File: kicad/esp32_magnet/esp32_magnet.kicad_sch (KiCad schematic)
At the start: 1 part, among them U1 ESP32-S3-WROOM-1

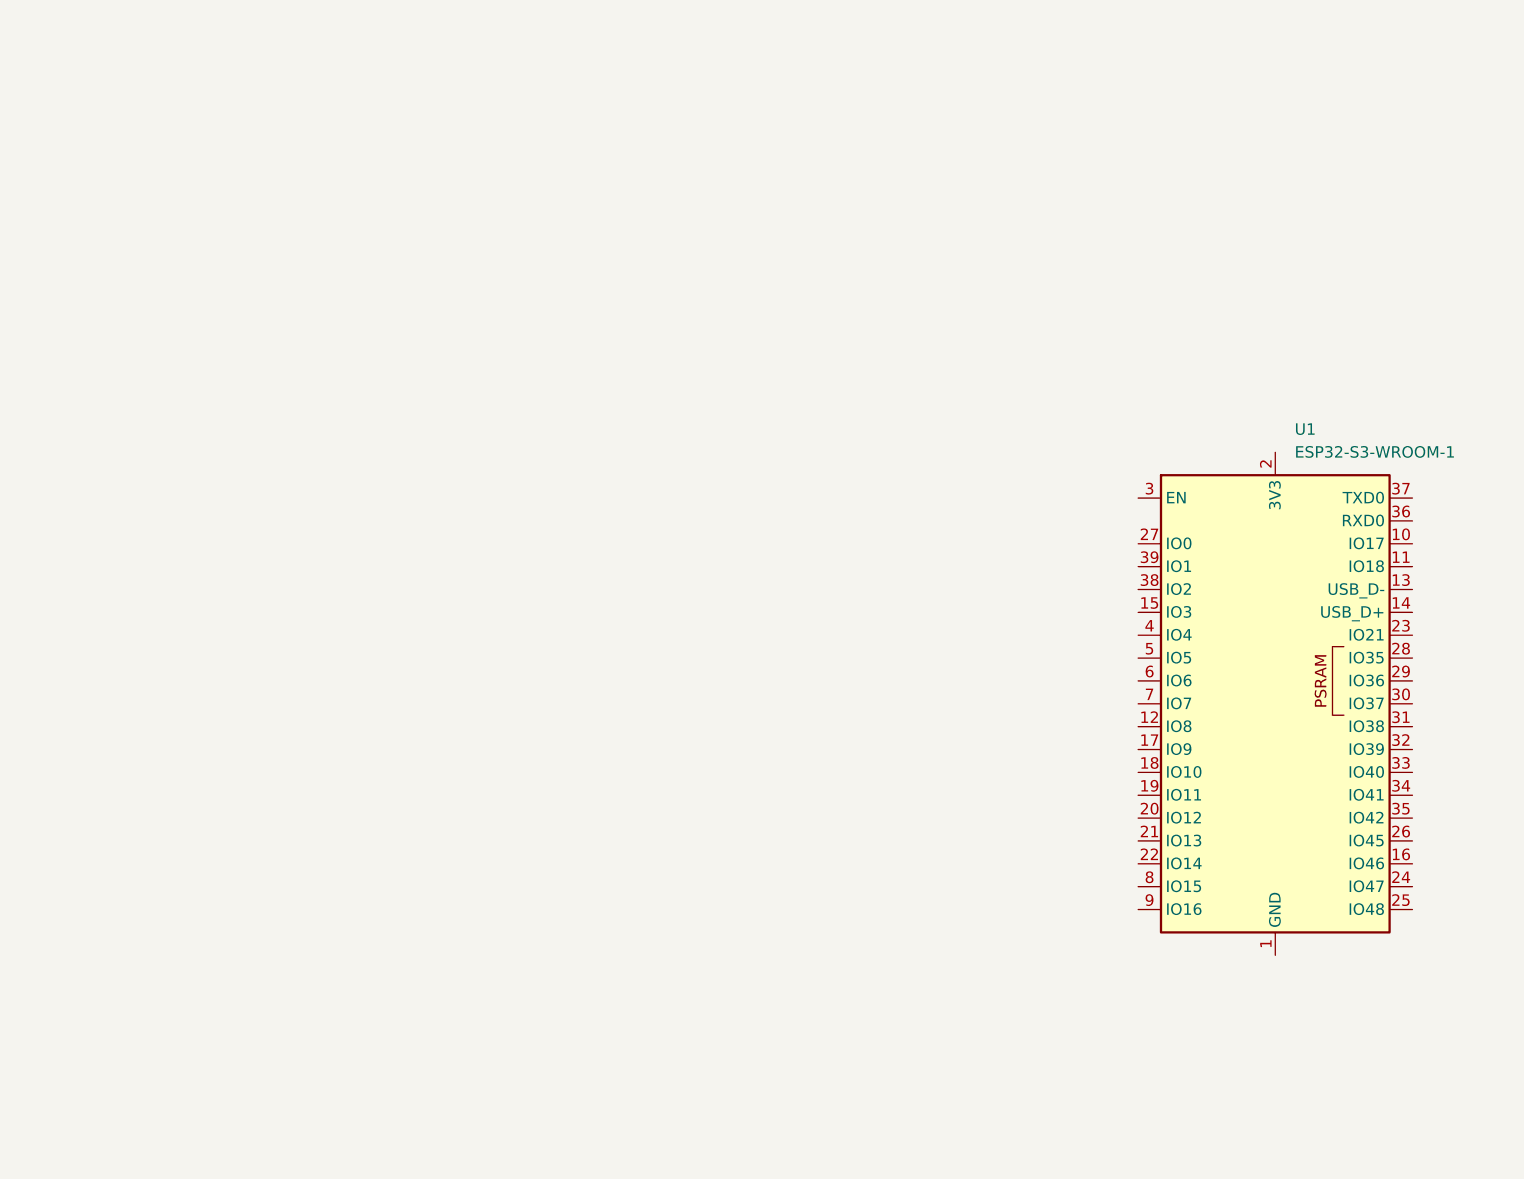
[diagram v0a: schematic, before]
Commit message: fix(kicad):esp32 base sch
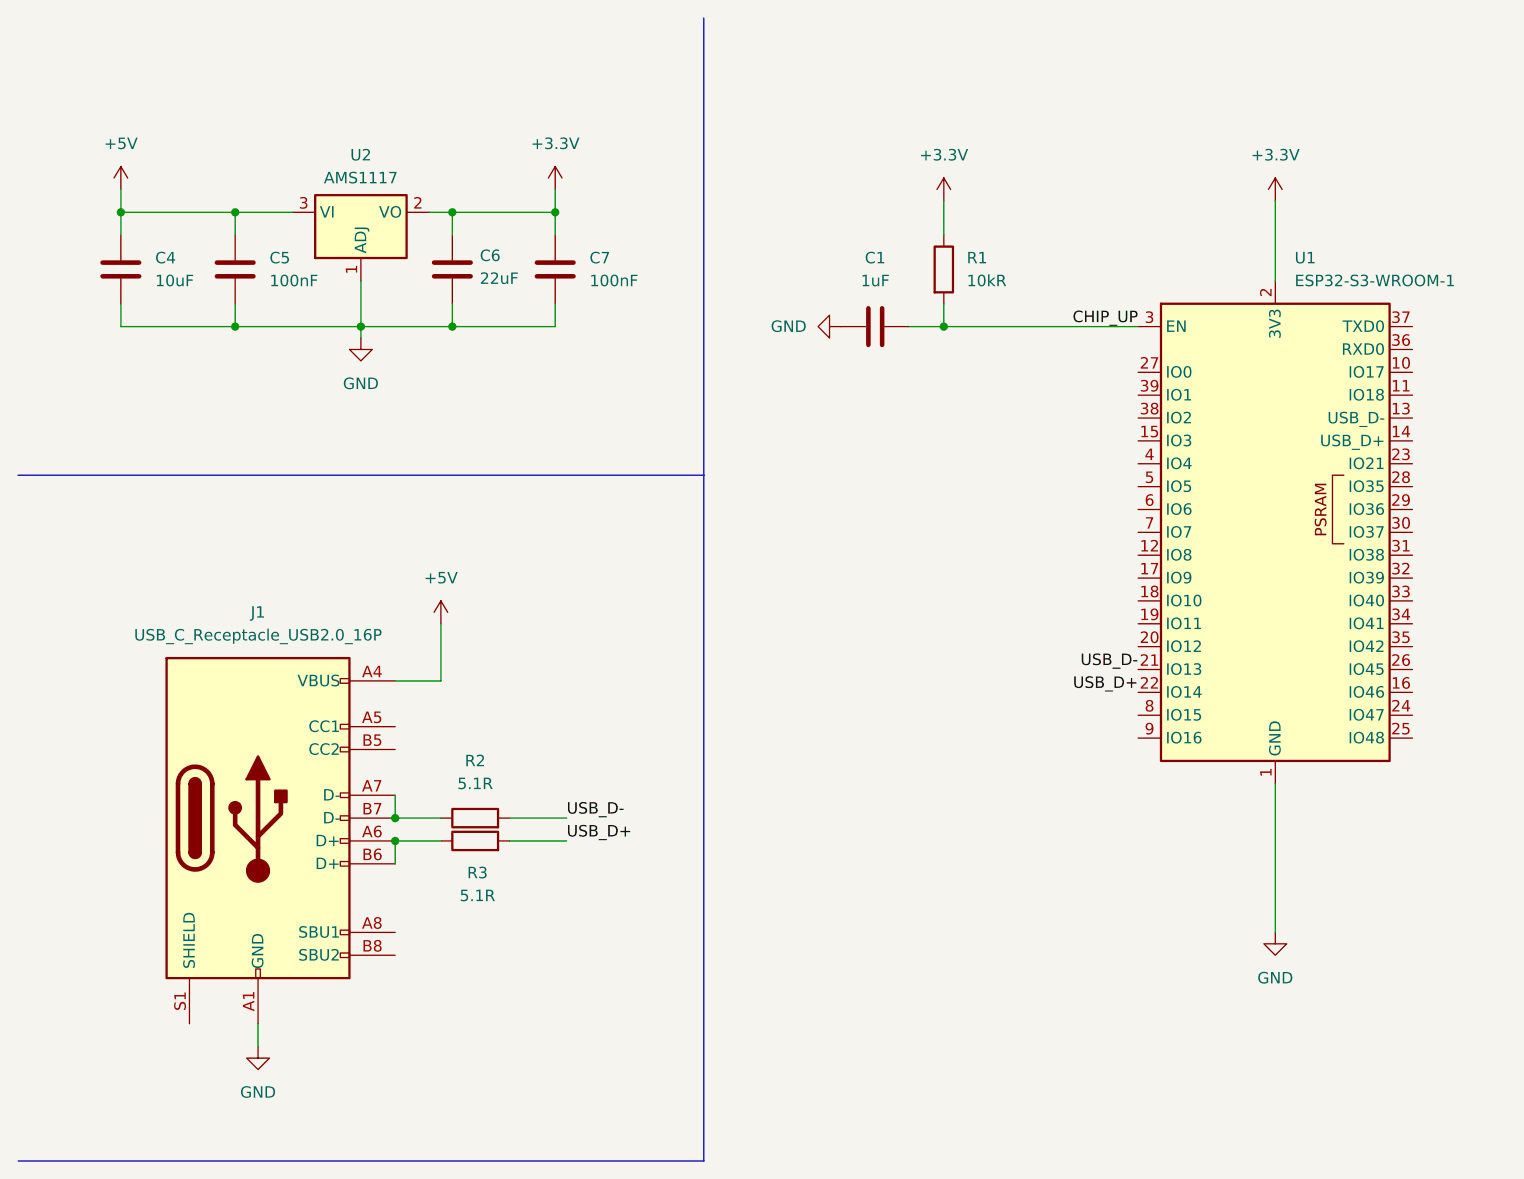
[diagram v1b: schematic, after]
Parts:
- added C1: 1uF, Capacitor_SMD:C_0603_1608Metric, symbol Device:C
- added C4: 10uF, Capacitor_SMD:C_0603_1608Metric, symbol Device:C
- added C5, C7: 100nF, Capacitor_SMD:C_0603_1608Metric, symbol Device:C
- added C6: 22uF, Capacitor_SMD:C_0603_1608Metric, symbol Device:C
- added J1: USB_C_Receptacle_USB2.0_16P, Connector_USB:USB_C_Receptacle_GCT_USB4105-xx-A_16P_TopMnt_Horizontal, symbol Connector:USB_C_Receptacle_USB2.0_16P
- added R1: 10kR, Resistor_SMD:R_1206_3216Metric, symbol Device:R
- added R2, R3: 5.1R, Resistor_SMD:R_1206_3216Metric, symbol Device:R
- added U2: AMS1117, Package_TO_SOT_SMD:SOT-223-3_TabPin2, symbol Regulator_Linear:AMS1117
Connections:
- net GND: now reaches U1.1 (GND), U1.40 (GND), U1.41 (GND)
- net GND: now also C1.1, C4.2, C5.2, C6.2, C7.2, J1.A1 (GND), J1.A12 (GND), J1.B1 (GND), J1.B12 (GND), U2.1 (ADJ)
- net +3.3V: now reaches U1.2 (3V3)
- net +3.3V: now also C6.1, C7.1, R1.1, U2.2 (VO)
- net USB_D-: now reaches U1.21 (IO13)
- net USB_D-: now also R2.2
- net USB_D+: now reaches U1.22 (IO14)
- net USB_D+: now also R3.2
- net CHIP_UP: now reaches U1.3 (EN)
- net CHIP_UP: now also C1.2, R1.2
- new net: J1.A6 (D+), J1.B6 (D+), R3.1
- new net: J1.A7 (D-), J1.B7 (D-), R2.1
- new net +5V: C4.1, C5.1, J1.A4 (VBUS), J1.A9 (VBUS), J1.B4 (VBUS), J1.B9 (VBUS), U2.3 (VI)
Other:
- moved on the sheet: U1

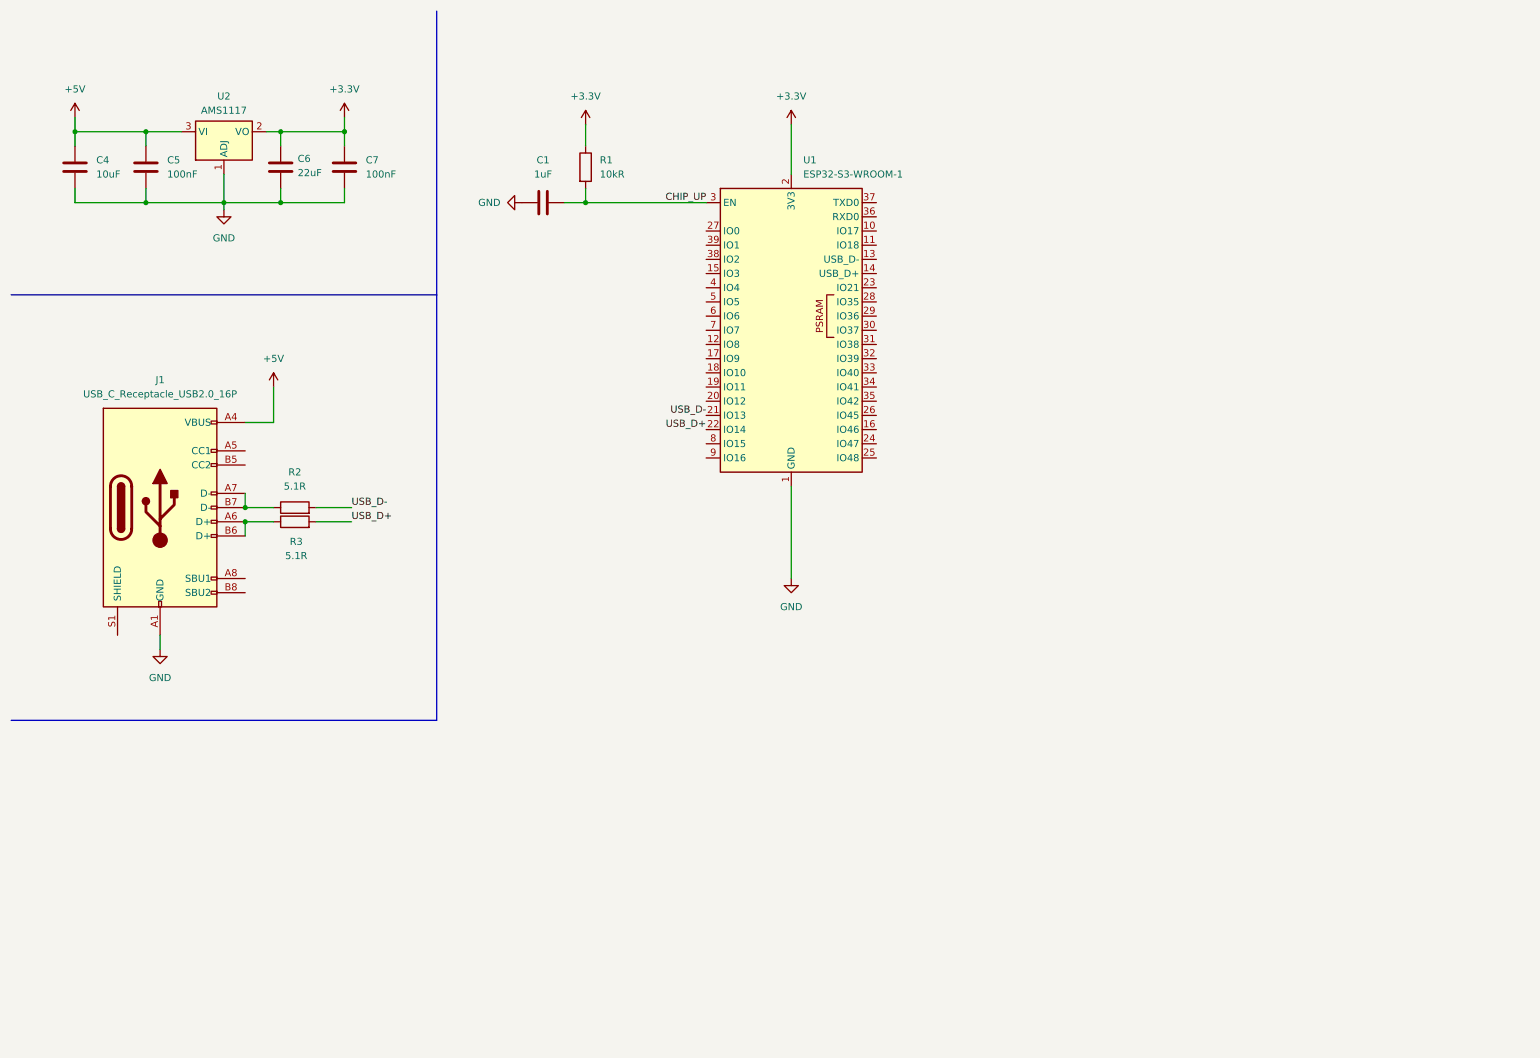
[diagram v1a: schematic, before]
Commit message: fix(kicad):esp32
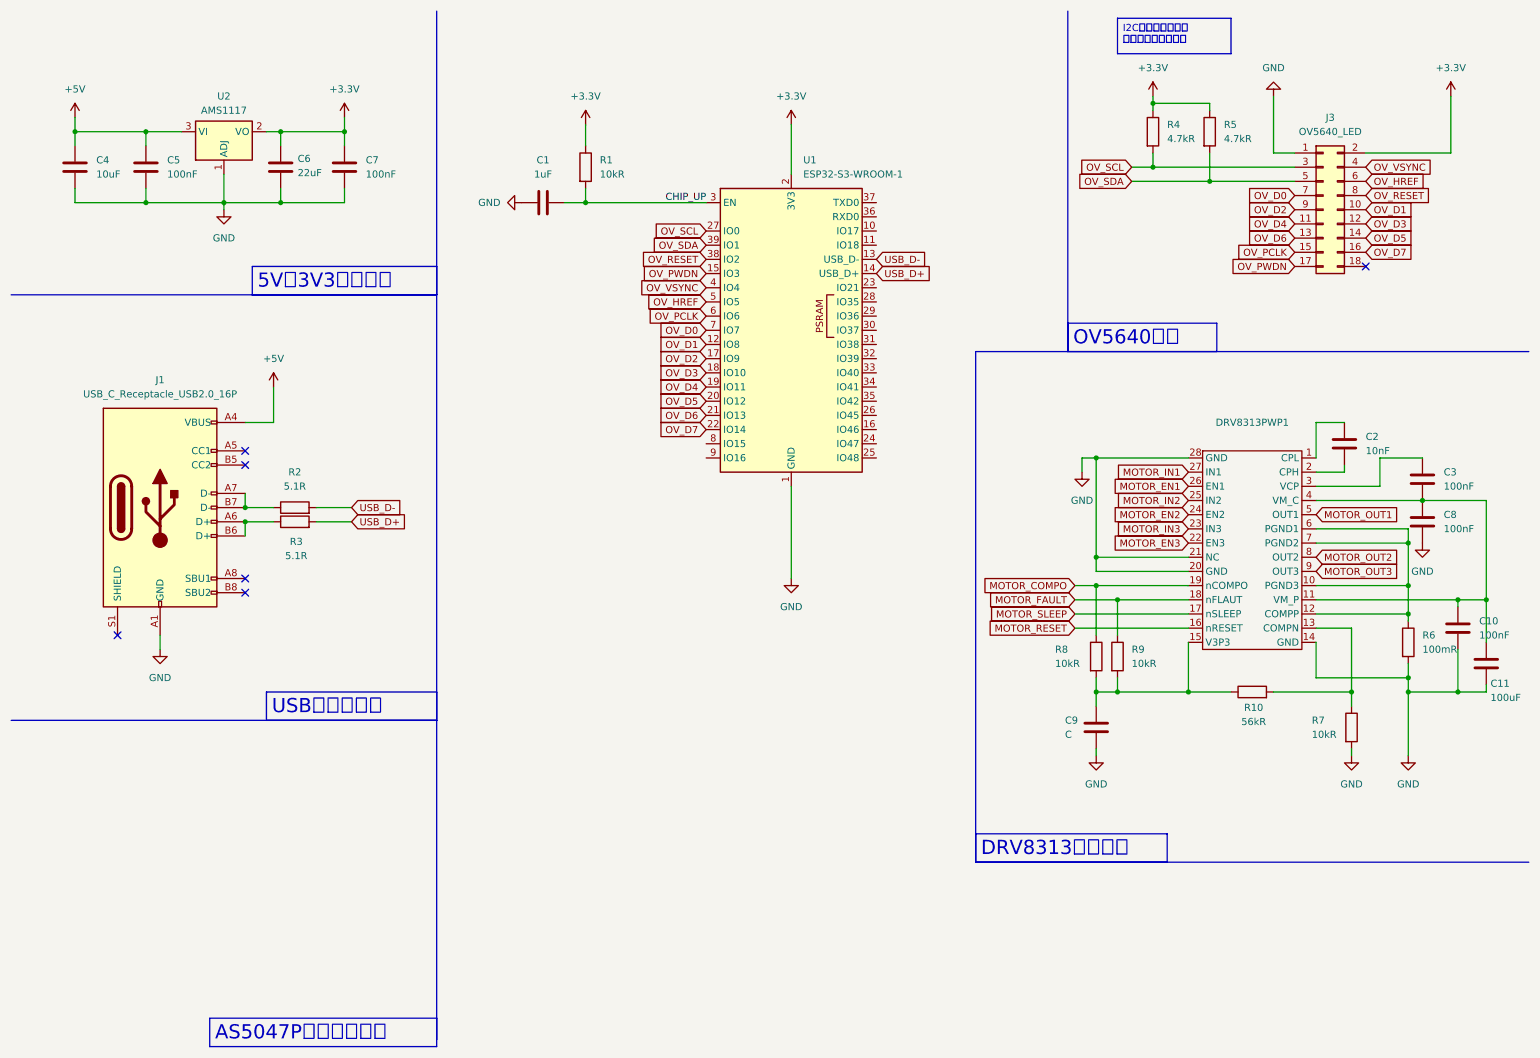
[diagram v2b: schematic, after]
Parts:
- added C10, C3, C8: 100nF, Capacitor_SMD:C_0603_1608Metric, symbol Device:C
- added C11: 100uF, Capacitor_SMD:C_1206_3216Metric, symbol Device:C
- added C2: 10nF, Capacitor_SMD:C_0603_1608Metric, symbol Device:C
- added C9: C, symbol Device:C
- added DRV8313PWP1: ~, DriverIC:DRV8313PWP-SOP65P640X120-29N, symbol DRV8313PWP:DRV8313PWP_0
- added J3: OV5640_LED, symbol Connector_Generic:Conn_02x09_Odd_Even
- added R10: 56kR, Resistor_SMD:R_1206_3216Metric, symbol Device:R
- added R4, R5: 4.7kR, symbol Device:R
- added R6: 100mR, Resistor_SMD:R_1206_3216Metric, symbol Device:R
- added R7, R8, R9: 10kR, Resistor_SMD:R_1206_3216Metric, symbol Device:R
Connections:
- net +3.3V: now also J3.2 (Pin_2), R4.1, R5.1
- net GND: now also C10.2, C11.2, C8.2, C9.2, DRV8313PWP1.14 (GND), DRV8313PWP1.20 (GND), DRV8313PWP1.21 (NC), DRV8313PWP1.28 (GND), J3.1 (Pin_1), R6.2, R7.2
- net USB_D+: now also U1.14 (USB_D+); no longer U1.22 (IO14)
- net USB_D-: now also U1.13 (USB_D-); no longer U1.21 (IO13)
- net OV_D1: now reaches U1.12 (IO8)
- net OV_D1: now also J3.10 (Pin_10)
- net OV_PWDN: now reaches U1.15 (IO3)
- net OV_PWDN: now also J3.17 (Pin_17)
- net OV_D2: now reaches U1.17 (IO9)
- net OV_D2: now also J3.9 (Pin_9)
- net OV_D3: now reaches U1.18 (IO10)
- net OV_D3: now also J3.12 (Pin_12)
- net OV_D4: now reaches U1.19 (IO11)
- net OV_D4: now also J3.11 (Pin_11)
- net OV_D5: now reaches U1.20 (IO12)
- net OV_D5: now also J3.14 (Pin_14)
- net OV_SCL: now reaches U1.27 (IO0)
- net OV_SCL: now also J3.3 (Pin_3), R4.2
- net OV_RESET: now reaches U1.38 (IO2)
- net OV_RESET: now also J3.8 (Pin_8)
- net OV_SDA: now reaches U1.39 (IO1)
- net OV_SDA: now also J3.5 (Pin_5), R5.2
- net OV_VSYNC: now reaches U1.4 (IO4)
- net OV_VSYNC: now also J3.4 (Pin_4)
- net OV_HREF: now reaches U1.5 (IO5)
- net OV_HREF: now also J3.6 (Pin_6)
- net OV_PCLK: now reaches U1.6 (IO6)
- net OV_PCLK: now also J3.15 (Pin_15)
- net OV_D0: now reaches U1.7 (IO7)
- net OV_D0: now also J3.7 (Pin_7)
- new net: C10.1, C11.1, C3.2, C8.1, DRV8313PWP1.11 (VM_P), DRV8313PWP1.4 (VM_C)
- new net: C2.1, DRV8313PWP1.1 (CPL)
- new net: C2.2, DRV8313PWP1.2 (CPH)
- new net: DRV8313PWP1.10 (PGND3), DRV8313PWP1.12 (COMPP), DRV8313PWP1.6 (PGND1), DRV8313PWP1.7 (PGND2), R6.1
- new net: C9.1, DRV8313PWP1.15 (V3P3), R10.1, R8.2, R9.2
- new net: DRV8313PWP1.13 (COMPN), R10.2, R7.1
- new net: C3.1, DRV8313PWP1.3 (VCP)
- new net MOTOR_COMPO: DRV8313PWP1.19 (nCOMPO), R8.1
- new net MOTOR_EN1: DRV8313PWP1.26 (EN1)
- new net MOTOR_EN2: DRV8313PWP1.24 (EN2)
- new net MOTOR_EN3: DRV8313PWP1.22 (EN3)
- new net MOTOR_FAULT: DRV8313PWP1.18 (nFLAUT), R9.1
- new net MOTOR_IN1: DRV8313PWP1.27 (IN1)
- new net MOTOR_IN2: DRV8313PWP1.25 (IN2)
- new net MOTOR_IN3: DRV8313PWP1.23 (IN3)
- new net MOTOR_OUT1: DRV8313PWP1.5 (OUT1)
- new net MOTOR_OUT2: DRV8313PWP1.8 (OUT2)
- new net MOTOR_OUT3: DRV8313PWP1.9 (OUT3)
- new net MOTOR_RESET: DRV8313PWP1.16 (nRESET)
- new net MOTOR_SLEEP: DRV8313PWP1.17 (nSLEEP)
- new net OV_D6: J3.13 (Pin_13), U1.21 (IO13)
- new net OV_D7: J3.16 (Pin_16), U1.22 (IO14)
- no-connect marks 0 -> 6
